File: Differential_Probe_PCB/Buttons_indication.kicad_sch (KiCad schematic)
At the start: 32 parts, among them Q101 AO3401A, Q102 AO3400A, SW101 TL2202EEYA, SW102 TL2202EEYA, U104 LM339

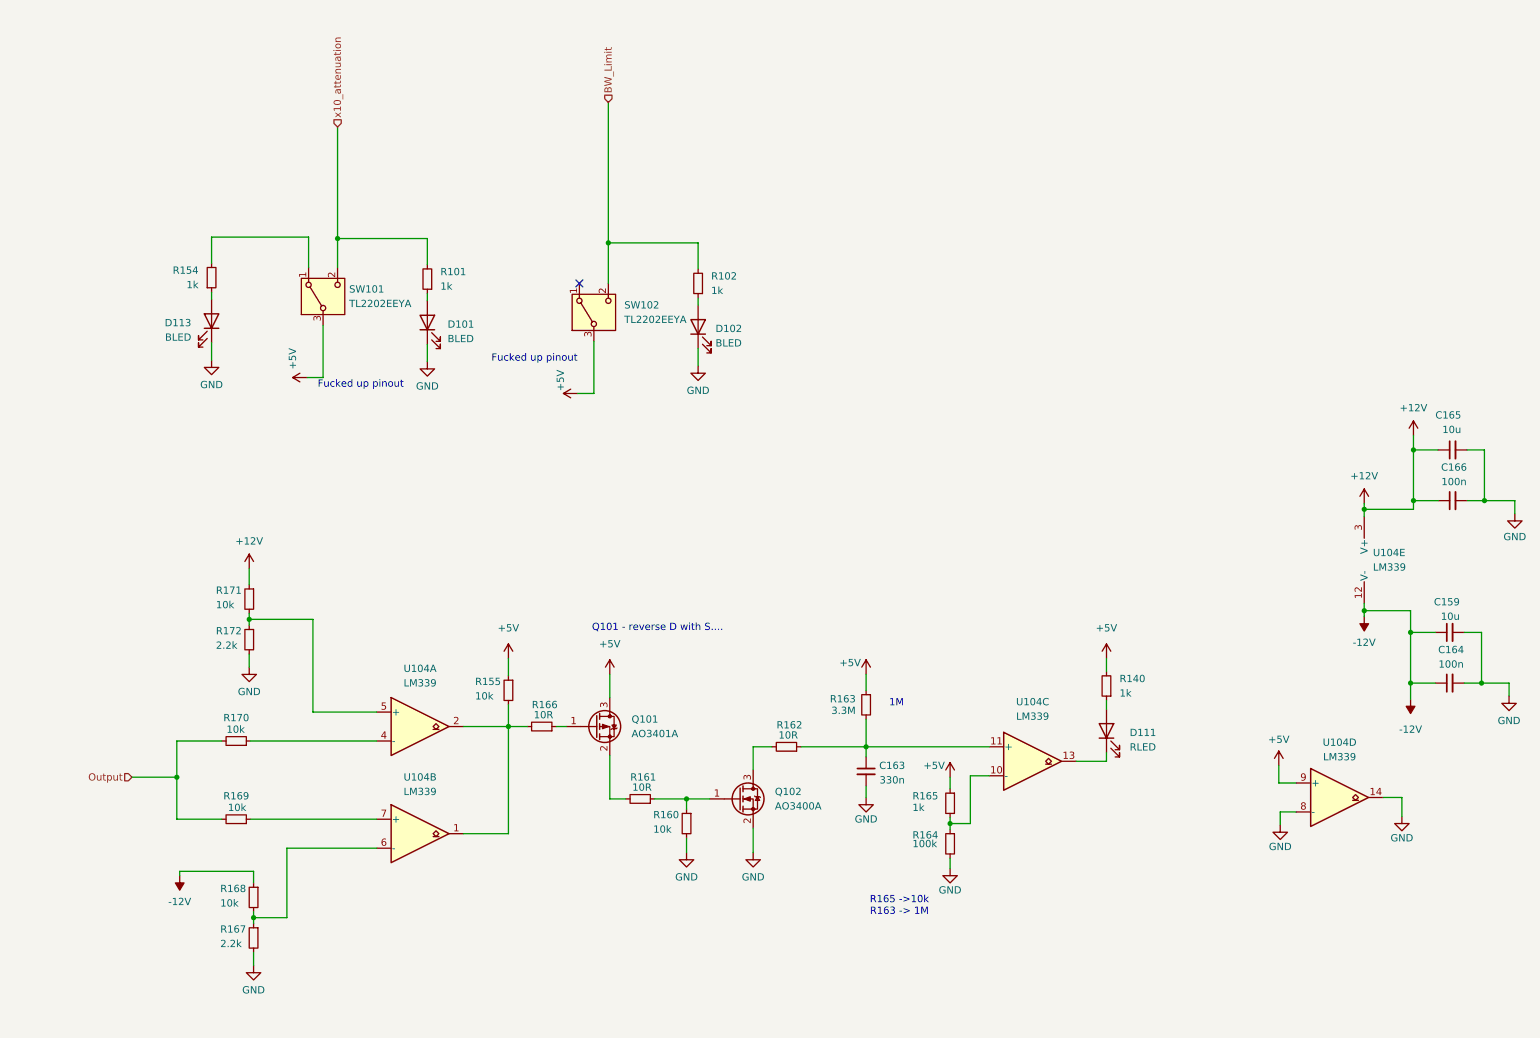
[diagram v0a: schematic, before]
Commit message: .
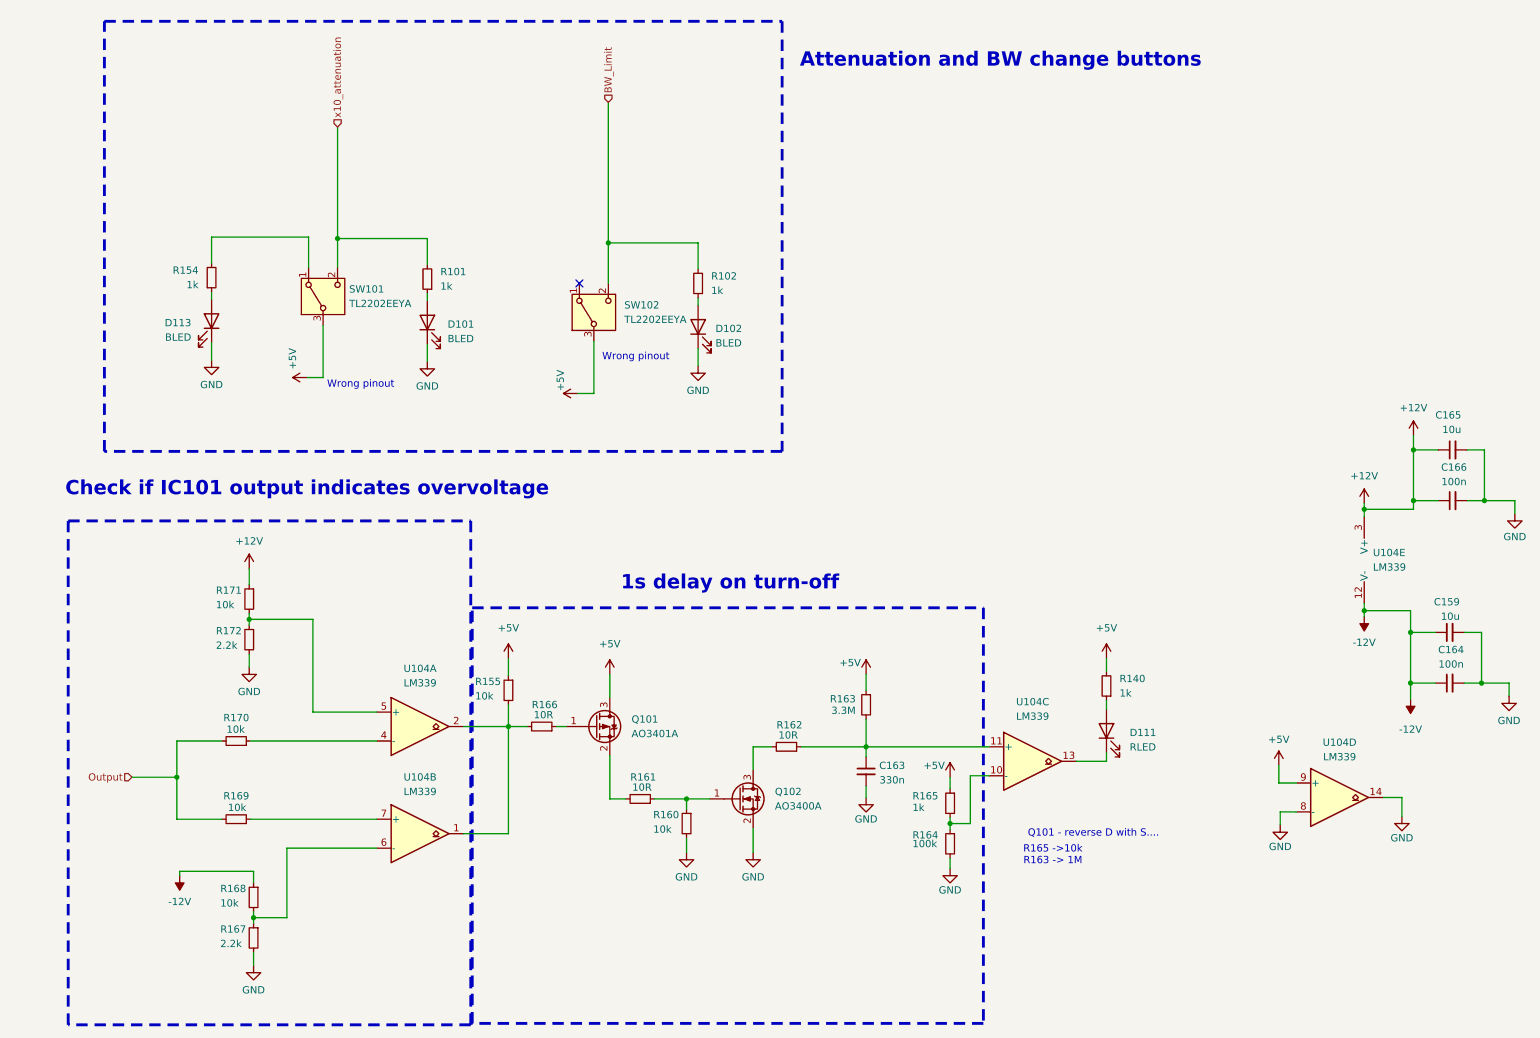
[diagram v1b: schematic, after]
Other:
- note added: "1s delay on turn-off"
- note added: "Attenuation and BW change buttons"
- note added: "Check if IC101 output indicates overvoltage"
- note added: "Wrong pinout"
- note removed: "1M"
- note removed: "Fucked up pinout"
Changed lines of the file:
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@@
 	(generator_version "9.0")
 	(paper "A4")
-	(text "Fucked up pinout"
+	(rectangle
+		(start 20.574 13.208)
+		(end 139.446 88.646)
+		(stroke
+			(width 0.5)
+			(type dash)
+		)
+		(fill
+			(type none)
+		)
+	)
+	(rectangle
+		(start 85.09 116.078)
+		(end 174.752 188.976)
+		(stroke
+			(width 0.5)
+			(type dash)
+		)
+		(fill
+			(type none)
+		)
+	)
+	(rectangle
+		(start 14.224 100.838)
+		(end 84.836 189.23)
+		(stroke
+			(width 0.5)
+			(type dash)
+		)
+		(fill
+			(type none)
+		)
+	)
+	(text "Check if IC101 output indicates overvoltage"
+		(exclude_from_sim no)
+		(at 56.134 95.25 0)
+		(effects
+			(font
+				(size 2.5 2.5)
+				(thickness 0.5)
+				(bold yes)
+			)
+		)
+	)
+	(text "Attenuation and BW change buttons"
+		(exclude_from_sim no)
+		(at 177.8 20.066 0)
+		(effects
+			(font
+				(size 2.5 2.5)
+				(thickness 0.5)
+				(bold yes)
+			)
+		)
+	)
+	(text "Wrong pinout"
 		(exclude_from_sim no)
 		(at 65.532 76.962 0)
@@
 		)
 	)
-	(text "Fucked up pinout"
+	(text "Wrong pinout"
 		(exclude_from_sim no)
-		(at 96.012 72.39 0)
+		(at 113.792 72.136 0)
 		(effects
 			(font
@@
 	(text "Q101 - reverse D with S...."
 		(exclude_from_sim no)
-		(at 117.602 119.634 0)
+		(at 194.056 155.702 0)
 		(effects
 			(font
@@
 		)
 	)
-	(text "1M\n"
+	(text "1s delay on turn-off"
 		(exclude_from_sim no)
-		(at 159.512 132.842 0)
+		(at 130.302 111.76 0)
 		(effects
 			(font
-				(size 1.27 1.27)
+				(size 2.5 2.5)
+				(thickness 0.5)
+				(bold yes)
 			)
 		)
@@
 	(text "R165 ->10k\nR163 -> 1M\n"
 		(exclude_from_sim no)
-		(at 160.02 168.402 0)
+		(at 186.944 159.512 0)
 		(effects
 			(font
